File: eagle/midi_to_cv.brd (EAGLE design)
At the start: 100 x 80 mm, 46 parts, among them IC2 4504N, IC3 4099N, U1 ATMEGA328P_PDIP

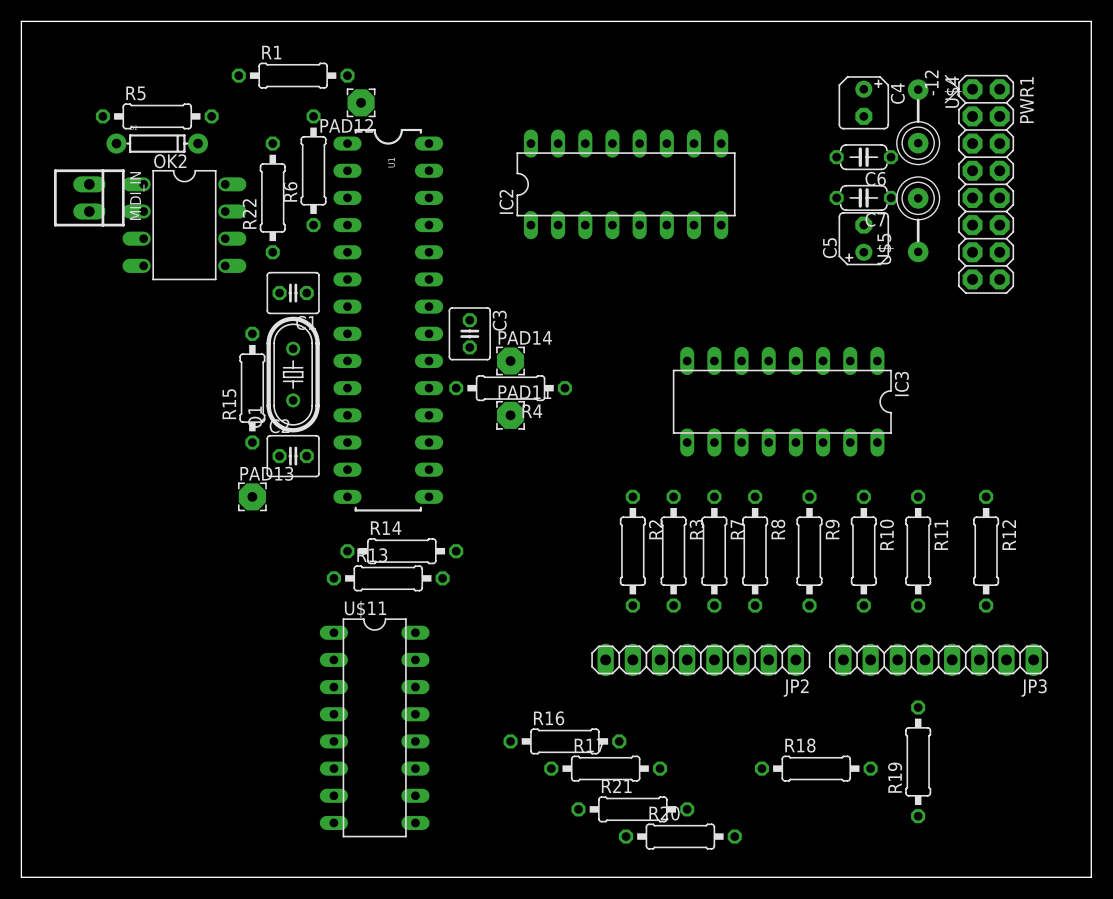
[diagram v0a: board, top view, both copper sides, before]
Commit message: a manual start
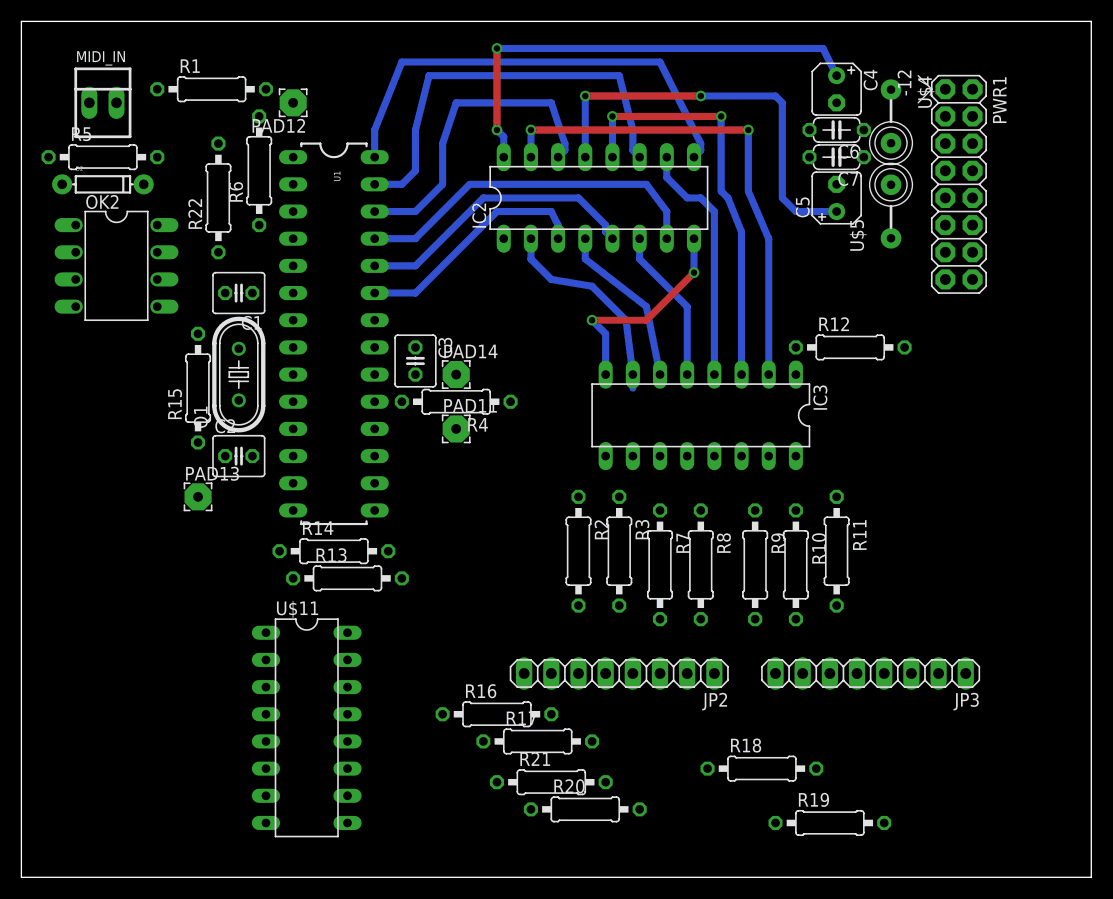
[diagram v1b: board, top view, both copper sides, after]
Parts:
- moved R12 22.9 mm to (77.5, 49.5), turned to 0 degrees
- moved R19 10.0 mm to (75.6, 5.08), turned to 0 degrees
- moved R20 9.25 mm to (52.7, 6.35)
- moved MIDI_IN 8.98 mm to (7.62, 72.4), turned to 0 degrees
- moved R21 8.03 mm to (49.5, 8.89)
- moved IC3 7.73 mm to (63.5, 43.2)
- moved R1 7.73 mm to (17.8, 73.7)
- moved JP2 7.73 mm to (55.9, 19.1)
- moved R11 7.62 mm to (76.2, 30.5)
- moved OK2 7.41 mm to (8.89, 57.1)
- moved R17 6.84 mm to (48.3, 12.7)
- moved R16 6.84 mm to (44.5, 15.2)
- moved JP3 6.48 mm to (79.4, 19.1)
- moved R10 6.48 mm to (72.4, 29.2)
- moved D2 6.35 mm to (7.62, 64.8)
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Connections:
- net N$13: now also U1.25; no longer U1.23
- net N$25: now also U1.23; no longer U1.25
- net N$37: now also IC3.4; no longer IC3.3
- net N$38: now also IC3.3; no longer IC3.4
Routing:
- net N$61: track 0.00 -> 46.1 mm, vias 0 -> 2
- net +12V: track 0.00 -> 43.7 mm, vias 0 -> 2
- net N$30: track 0.00 -> 43.6 mm
- net N$32: track 0.00 -> 39.2 mm
- net +5V: track 0.00 -> 38.9 mm, vias 0 -> 2
- net N$38: track 0.00 -> 38.6 mm, vias 0 -> 2
- net N$13: track 0.00 -> 33.2 mm
- net N$31: track 0.00 -> 29.7 mm
- net N$23: track 0.00 -> 26.8 mm
- net N$37: track 0.00 -> 22.9 mm
- net N$25: track 0.00 -> 22.4 mm
- net GND: track 0.00 -> 20.1 mm, vias 0 -> 2
- net N$36: track 0.00 -> 19.3 mm
- net N$35: track 0.00 -> 15.6 mm
- net N$33: track 0.00 -> 14.5 mm
